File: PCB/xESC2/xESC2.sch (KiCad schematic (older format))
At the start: 0 parts

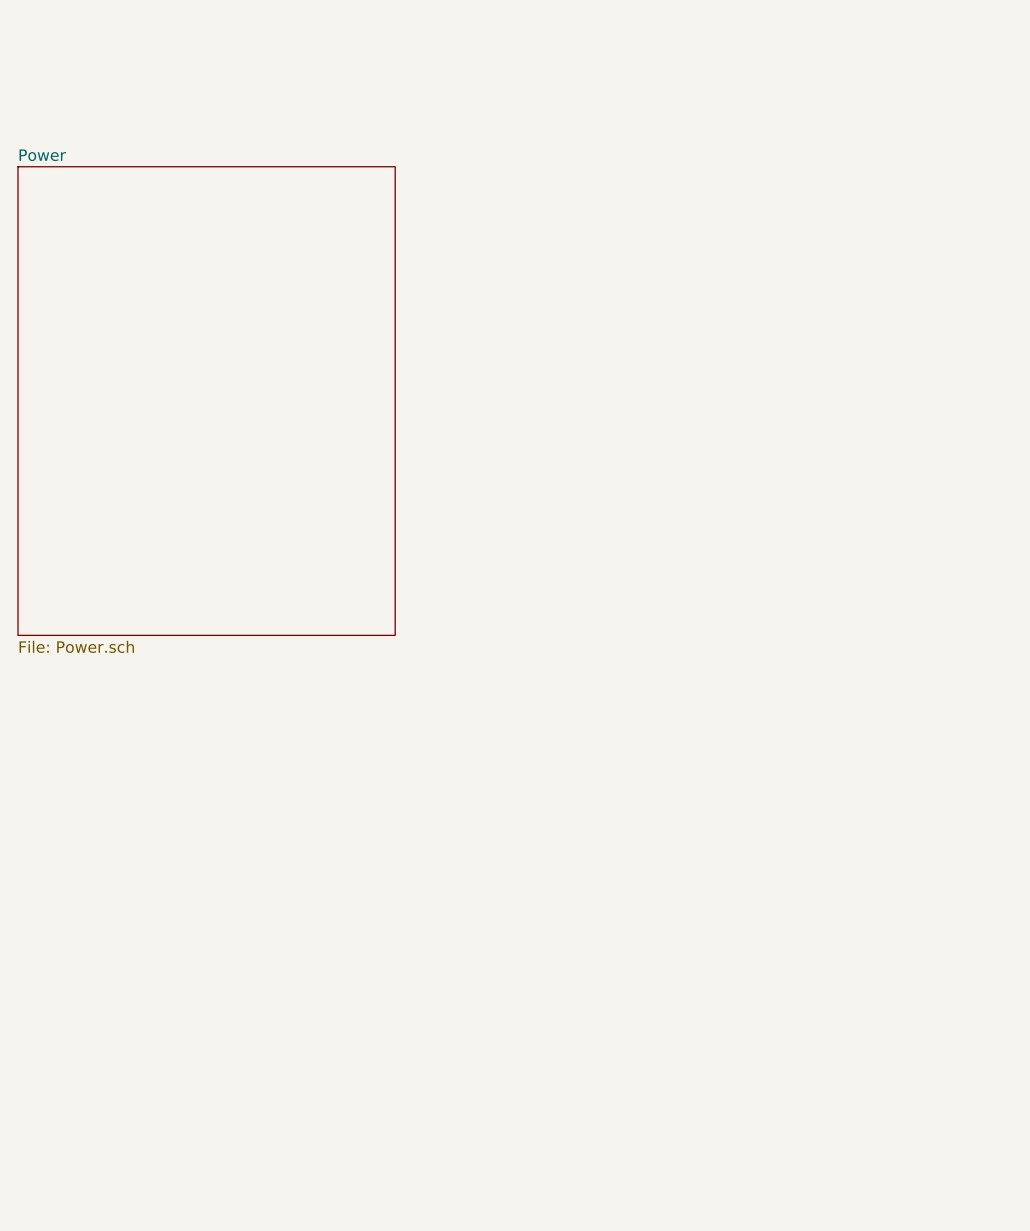
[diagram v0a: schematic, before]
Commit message: wip
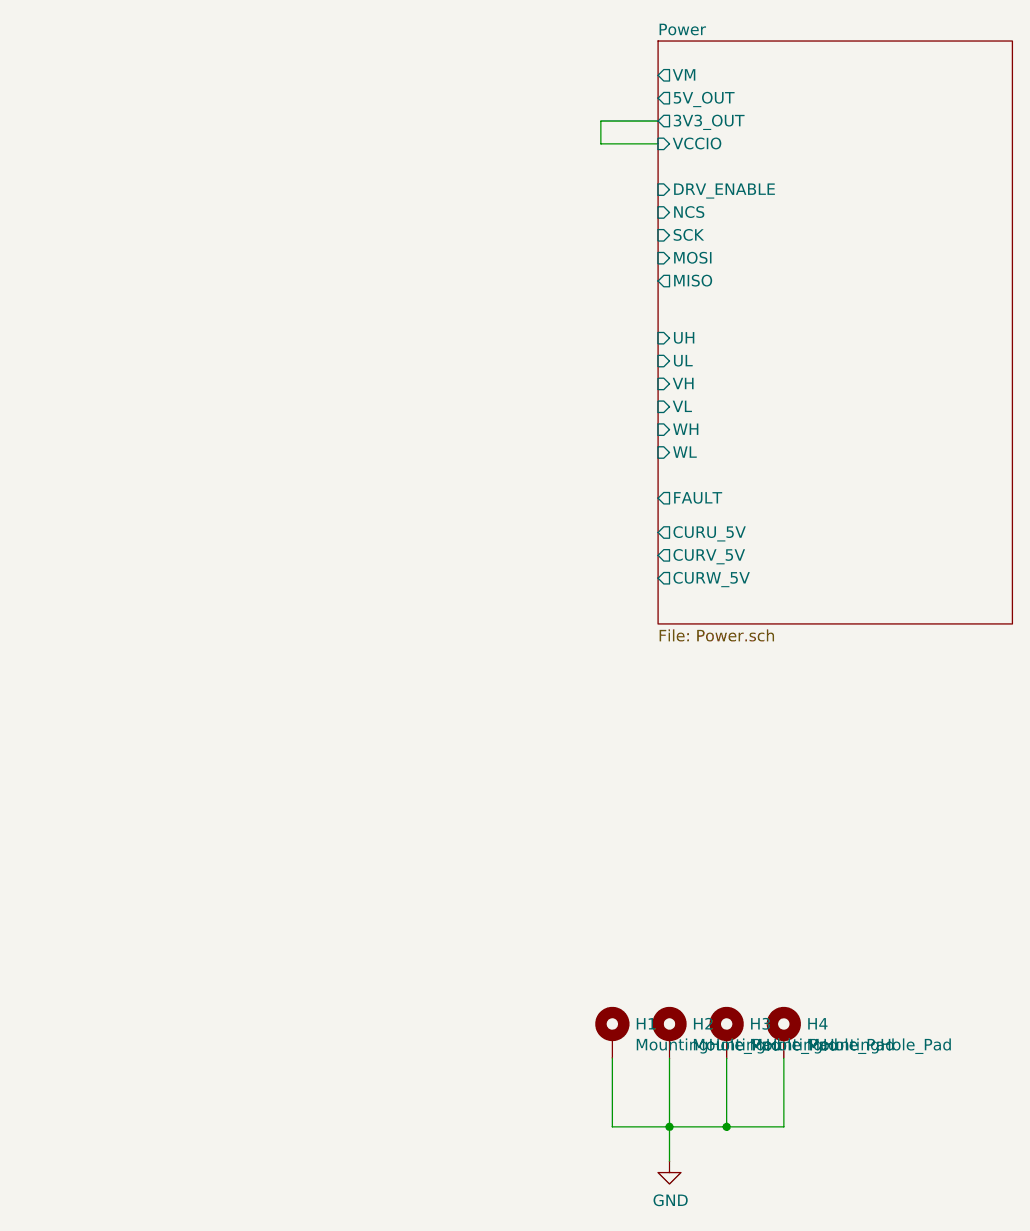
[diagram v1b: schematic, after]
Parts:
- added H1, H2, H3, H4: MountingHole_Pad, MountingHole:MountingHole_2.7mm_M2.5_DIN965_Pad, symbol Mechanical:MountingHole_Pad
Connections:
- new net GND: H1.1, H2.1, H3.1, H4.1
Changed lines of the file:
@@
 $EndDescr
 $Sheet
-S 6000 1950 1650 2050
+S 8800 1400 1550 2550
 U 61A3F4E8
 F0 "Power" 50
 F1 "Power.sch" 50
+F2 "DRV_ENABLE" I L 8800 2050 50
+F3 "NCS" I L 8800 2150 50
+F4 "SCK" I L 8800 2250 50
+F5 "MOSI" I L 8800 2350 50
+F6 "MISO" O L 8800 2450 50
+F7 "UH" I L 8800 2700 50
+F8 "UL" I L 8800 2800 50
+F9 "VH" I L 8800 2900 50
+F10 "VL" I L 8800 3000 50
+F11 "WH" I L 8800 3100 50
+F12 "WL" I L 8800 3200 50
+F13 "FAULT" O L 8800 3400 50
+F14 "CURU_5V" O L 8800 3550 50
+F15 "CURV_5V" O L 8800 3650 50
+F16 "CURW_5V" O L 8800 3750 50
+F17 "VCCIO" I L 8800 1850 50
+F18 "5V_OUT" O L 8800 1650 50
+F19 "3V3_OUT" O L 8800 1750 50
+F20 "VM" O L 8800 1550 50
 $EndSheet
+Wire Wire Line
+	8800 1750 8550 1750
+Wire Wire Line
+	8550 1750 8550 1850
+Wire Wire Line
+	8550 1850 8800 1850
+$Comp
+L Mechanical:MountingHole_Pad H1
+U 1 1 61DB61D0
+P 8600 5750
+F 0 "H1" H 8700 5799 50  0000 L CNN
+F 1 "MountingHole_Pad" H 8700 5708 50  0000 L CNN
+F 2 "MountingHole:MountingHole_2.7mm_M2.5_DIN965_Pad" H 8600 5750 50  0001 C CNN
+F 3 "~" H 8600 5750 50  0001 C CNN
+	1    8600 5750
+	1    0    0    -1
+$EndComp
+$Comp
+L Mechanical:MountingHole_Pad H2
+U 1 1 61DB6764
+P 8850 5750
+F 0 "H2" H 8950 5799 50  0000 L CNN
+F 1 "MountingHole_Pad" H 8950 5708 50  0000 L CNN
+F 2 "MountingHole:MountingHole_2.7mm_M2.5_DIN965_Pad" H 8850 5750 50  0001 C CNN
+F 3 "~" H 8850 5750 50  0001 C CNN
+	1    8850 5750
+	1    0    0    -1
+$EndComp
+$Comp
+L Mechanical:MountingHole_Pad H3
+U 1 1 61DB6A4D
+P 9100 5750
+F 0 "H3" H 9200 5799 50  0000 L CNN
+F 1 "MountingHole_Pad" H 9200 5708 50  0000 L CNN
+F 2 "MountingHole:MountingHole_2.7mm_M2.5_DIN965_Pad" H 9100 5750 50  0001 C CNN
+F 3 "~" H 9100 5750 50  0001 C CNN
+	1    9100 5750
+	1    0    0    -1
+$EndComp
+$Comp
+L Mechanical:MountingHole_Pad H4
+U 1 1 61DB6BE9
+P 9350 5750
+F 0 "H4" H 9450 5799 50  0000 L CNN
+F 1 "MountingHole_Pad" H 9450 5708 50  0000 L CNN
+F 2 "MountingHole:MountingHole_2.7mm_M2.5_DIN965_Pad" H 9350 5750 50  0001 C CNN
+F 3 "~" H 9350 5750 50  0001 C CNN
+	1    9350 5750
+	1    0    0    -1
+$EndComp
+Wire Wire Line
+	8600 5850 8600 6150
+Wire Wire Line
+	8600 6150 8850 6150
+Wire Wire Line
+	9350 6150 9350 5850
+Wire Wire Line
+	9100 5850 9100 6150
+Connection ~ 9100 6150
+Wire Wire Line
+	9100 6150 9350 6150
+Wire Wire Line
+	8850 6150 8850 5850
+Connection ~ 8850 6150
+Wire Wire Line
+	8850 6150 9100 6150
+$Comp
+L power:GND #PWR0119
+U 1 1 61DB7185
+P 8850 6300
+F 0 "#PWR0119" H 8850 6050 50  0001 C CNN
+F 1 "GND" H 8855 6127 50  0000 C CNN
+F 2 "" H 8850 6300 50  0001 C CNN
+F 3 "" H 8850 6300 50  0001 C CNN
+	1    8850 6300
+	1    0    0    -1
+$EndComp
+Wire Wire Line
+	8850 6300 8850 6150
 $EndSCHEMATC
